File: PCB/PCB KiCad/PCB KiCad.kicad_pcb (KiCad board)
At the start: 2 copper layers, 40 x 40 mm, 54 parts, among them J1 Conn_01x04, J2 Qwiic, J3 Conn_01x04, J4 Conn_01x04, J5 Conn_01x04, U1 OPA2376AID, U2 NAU7802SGI, U3 TLC59208FIPWR, U4 LP5951MFX-1.8_NOPB

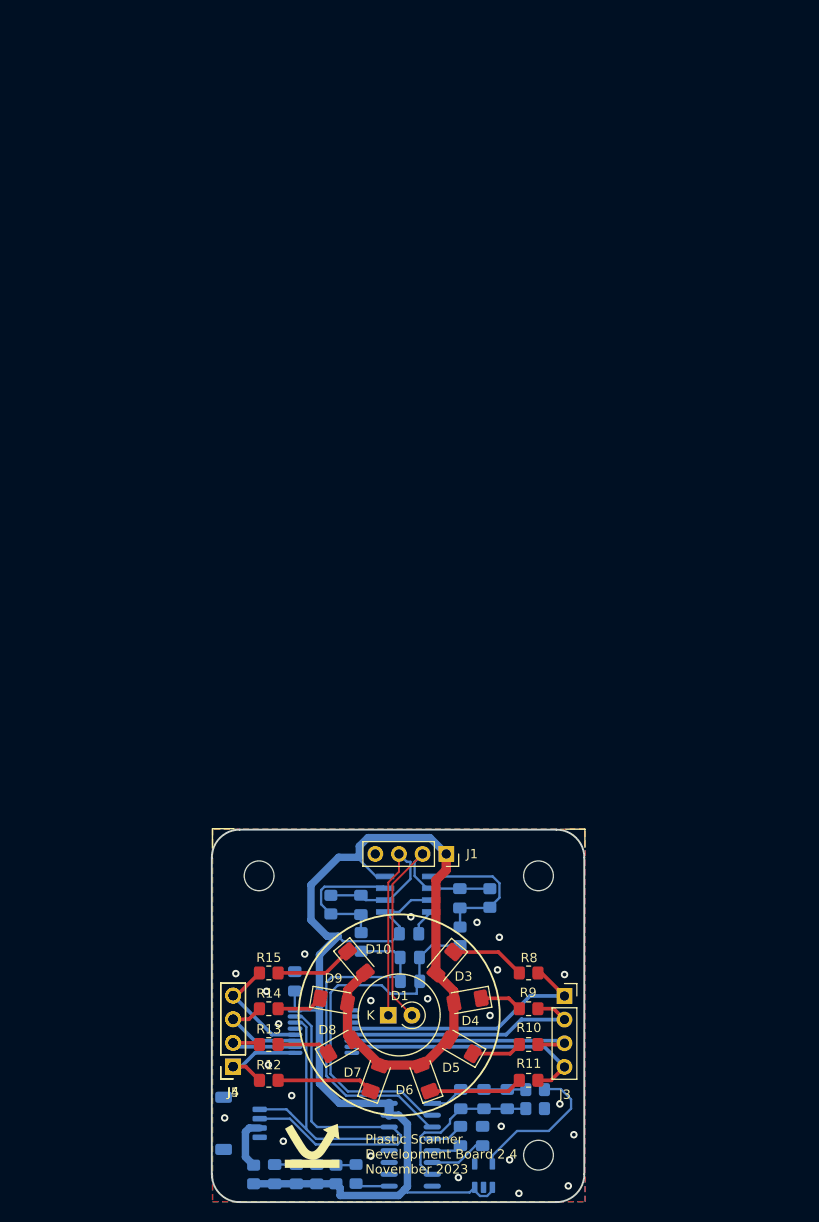
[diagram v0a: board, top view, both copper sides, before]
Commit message: Minor schematic cleanup!
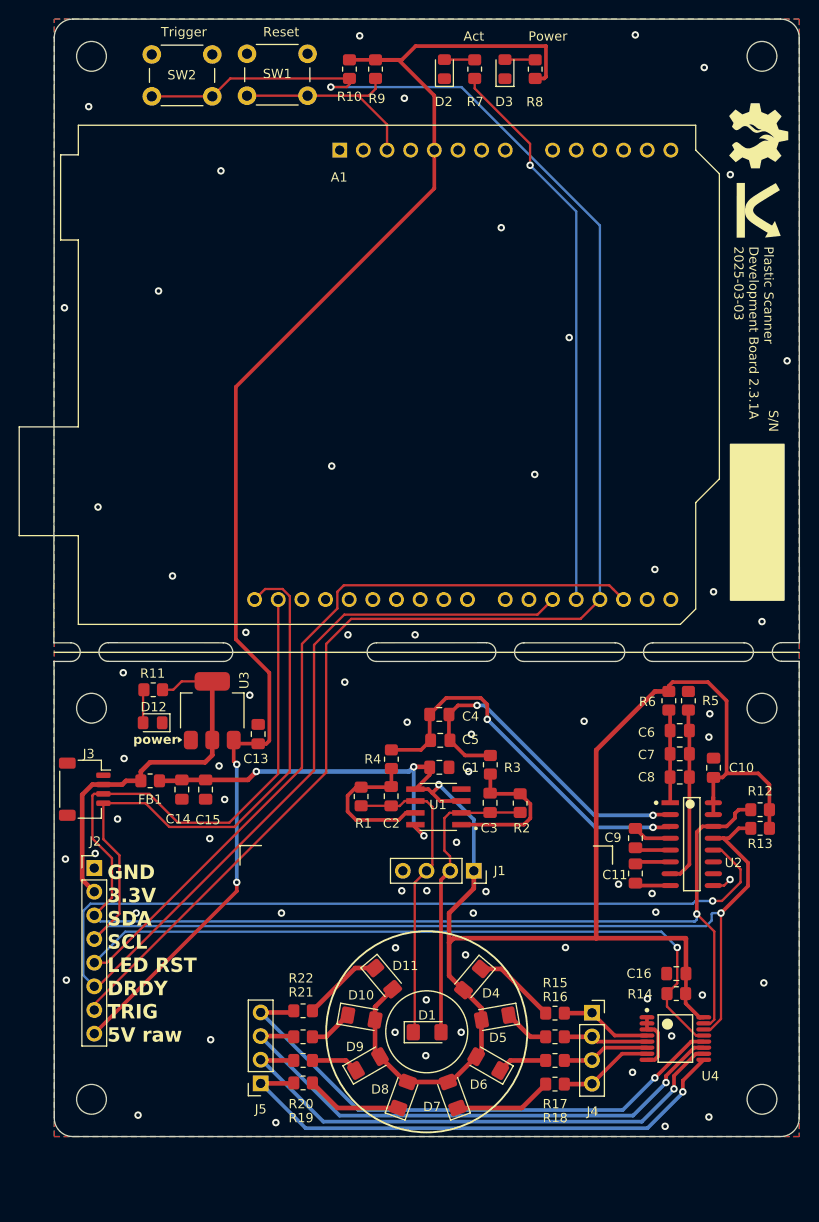
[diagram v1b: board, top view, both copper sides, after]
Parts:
- removed the C14 at (68.8, 131.3)
- removed the D10 at (75.4, 129.3)
- removed H1, H2, H4: MountingHole, MountingHole:MountingHole_3.2mm_M3
- removed the J4 at (62.2, 140.5)
- removed the R11 at (93.9, 142.0)
- removed the R15 at (66.0, 130.4)
- added ?: MountingHole_3.2mm_M3, MountingHole:MountingHole_3.2mm_M3, F.Cu at (119.0, 32.0)
- added ?: MountingHole_3.2mm_M3, MountingHole:MountingHole_3.2mm_M3, F.Cu at (47.0, 144.0)
- added A1: Arduino_UNO_R3, Module:Arduino_UNO_R3, F.Cu at (73.7, 42.1)
- added C15: 22u, Capacitor_SMD:C_0805_2012Metric_Pad1.18x1.45mm_HandSolder, F.Cu at (59.2, 110.7)
- added C16: 100n, Capacitor_SMD:C_0805_2012Metric_Pad1.18x1.45mm_HandSolder, F.Cu at (109.8, 130.5)
- added D11: 1720nm, LED_SMD:LED_1206_3216Metric_Pad1.42x1.75mm_HandSolder, F.Cu at (78.4, 131.0)
- added D12: LED RED, LED_SMD:LED_0805_2012Metric_Pad1.15x1.40mm_HandSolder, F.Cu at (53.6, 103.6)
- added D3: LED RED, LED_SMD:LED_0805_2012Metric_Pad1.15x1.40mm_HandSolder, F.Cu at (91.4, 33.4)
- added G***: LOGO, LOGO, F.Cu at (118.9, 48.5)
- added G***: LOGO, LOGO, F.Cu at (118.6, 40.5)
- added G***: LOGO, LOGO, B.Cu at (83.4, 121.0)
- added G1: LOGO, LOGO, B.Cu at (82.0, 66.0)
- added J2: Conn_01x08, Connector_PinHeader_2.54mm:PinHeader_1x08_P2.54mm_Vertical, F.Cu at (47.3, 119.2)
- added R16: 47, Resistor_SMD:R_0805_2012Metric_Pad1.20x1.40mm_HandSolder, F.Cu at (96.8, 137.3)
- added R17: 47, Resistor_SMD:R_0805_2012Metric_Pad1.20x1.40mm_HandSolder, F.Cu at (96.8, 139.8)
- added R18: 47, Resistor_SMD:R_0805_2012Metric_Pad1.20x1.40mm_HandSolder, F.Cu at (96.8, 142.4)
- added R19: 47, Resistor_SMD:R_0805_2012Metric_Pad1.20x1.40mm_HandSolder, F.Cu at (69.7, 142.2)
- added R20: 47, Resistor_SMD:R_0805_2012Metric_Pad1.20x1.40mm_HandSolder, F.Cu at (69.7, 139.8)
- added R21: 47, Resistor_SMD:R_0805_2012Metric_Pad1.20x1.40mm_HandSolder, F.Cu at (69.7, 137.3)
- added R22: 47, Resistor_SMD:R_0805_2012Metric_Pad1.20x1.40mm_HandSolder, F.Cu at (69.7, 134.5)
- added R7: 100, Resistor_SMD:R_0805_2012Metric_Pad1.20x1.40mm_HandSolder, F.Cu at (88.2, 33.4)
- added R8: 100, Resistor_SMD:R_0805_2012Metric_Pad1.20x1.40mm_HandSolder, F.Cu at (94.7, 33.4)
- added REF**: MountingHole_3.2mm_M3, MountingHole:MountingHole_3.2mm_M3, F.Cu at (47.0, 32.0)
- added SW1: MCU_RESET, Button_Switch_THT:SW_PUSH_6mm, F.Cu at (63.7, 31.7)
- added SW2: TRIGGER, Button_Switch_THT:SW_PUSH_6mm, F.Cu at (53.5, 31.8)
- added e: MountingHole_3.2mm_M3, MountingHole:MountingHole_3.2mm_M3, F.Cu at (47.0, 102.0)
- added e: MountingHole_3.2mm_M3, MountingHole:MountingHole_3.2mm_M3, F.Cu at (119.0, 144.0)
- added e: MountingHole_3.2mm_M3, MountingHole:MountingHole_3.2mm_M3, F.Cu at (119.0, 102.0)
- C1, C10, C11, C2, C3, C4, C5, C6, C7, C8, C9, FB1, R1, R2, R3, R4, R5, R6, U1, U2: moved to F.Cu
- C13: value 22u -> 10u; moved to F.Cu
- C14: renamed from C12; moved to F.Cu
- D1: footprint Diode_THT:D_A-405_P2.54mm_Vertical_KathodeUp -> Diode_SMD:D_1206_3216Metric_Pad1.42x1.75mm_HandSolder
- D2: value LED RED -> LED BLUE; moved to F.Cu
- G***: moved to B.Cu
- J3: renamed from J2; moved to F.Cu
- R10, R9: value 47 -> 10k
- R11: renamed from R7; moved to F.Cu
- R12, R13: value 47 -> 4.7k
- R14: value 47 -> 1k
- U3: value TLC59208FIPWR -> AMS1117-3.3; footprint TLC59208:Texas_Instruments-TLC59208FIPWR-Level_A -> Package_TO_SOT_SMD:SOT-223-3_TabPin2; moved to F.Cu
- U4: value LP5951MFX-1.8_NOPB -> TLC59208FIPWR; footprint LP5951MFX-1.8_NOPB:SOT95P280X145-5N -> TLC59208:Texas_Instruments-TLC59208FIPWR-Level_A; moved to F.Cu
- moved D2 119.0 mm to (84.9, 33.4)
- moved R10 106.5 mm to (74.7, 33.4), turned to -90 degrees
- moved R9 102.2 mm to (77.5, 33.4), turned to -90 degrees
- moved C10 64.2 mm to (113.8, 108.4)
- moved R12 60.2 mm to (118.8, 112.9), turned to 180 degrees
- moved R13 57.6 mm to (118.8, 114.9), turned to 180 degrees
- moved R11 55.6 mm to (53.6, 100.0), turned to 180 degrees
- moved G*** 52.4 mm to (98.1, 104.1), turned to 180 degrees
- moved C13 47.4 mm to (64.9, 104.8)
- moved G*** 47.2 mm to (106.4, 104.3)
- moved R5 46.8 mm to (111.1, 101.2), turned to 90 degrees
- moved U2 44.2 mm to (111.5, 116.6), turned to 0 degrees
- moved R6 44.2 mm to (109.0, 101.2), turned to 90 degrees
- moved R14 43.8 mm to (109.8, 132.7)
- moved C14 43.8 mm to (56.7, 110.7), turned to 90 degrees
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- renumbered D9 to D10, D3 to D4, D4 to D5, D5 to D6, D6 to D7, D7 to D8, D8 to D9, J3 to J4, R8 to R15
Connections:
- C1 pad 2: 3.3v -> +3.3V
- C10 pad 1: 3.3v -> +3.3V
- C13 pad 1: 3.3v -> 5v_RAW
- C14 pad 2: 3.3v -> +3.3V
- D10 pad 1: Net-(D9-K) -> Net-(D10-K)
- D10 pad 2: 3.3v -> +3.3V
- D4 pad 2: 3.3v -> +3.3V
- D5 pad 1: Net-(D4-K) (its old number) -> Net-(D5-K)
- D5 pad 2: 3.3v -> +3.3V
- D6 pad 1: Net-(D5-K) -> Net-(D6-K)
- D6 pad 2: 3.3v -> +3.3V
- D7 pad 2: 3.3v -> +3.3V
- D8 pad 1: Net-(D7-K) (its old number) -> Net-(D8-K)
- D8 pad 2: 3.3v -> +3.3V
- D9 pad 1: Net-(D8-K) -> Net-(D9-K)
- D9 pad 2: 3.3v -> +3.3V
- FB1 pad 1: 3.3v -> +3.3V
- J1 pad 1: 3.3v -> +3.3V
- R10 pad 1: LED3 -> 5v_RAW
- R10 pad 2: Net-(D5-K) -> TRIGGER
- R11 pad 1: 3.3v -> 3v3unf
- R11 pad 2: Net-(D2-A) -> Net-(D12-A)
- R12 pad 1: LED5 -> +3.3V
- R12 pad 2: Net-(D7-K) (its old number) -> SDA
- R13 pad 1: LED6 -> +3.3V
- R13 pad 2: Net-(D8-K) -> SCL
- R14 pad 1: LED7 -> LED_RESET
- R14 pad 2: Net-(D9-K) -> +3.3V
- R6 pad 2: Net-(U4-VOUT) -> +3.3V
- R9 pad 1: LED2 -> 5v_RAW
- R9 pad 2: Net-(D4-K) (its old number) -> MCU_RESET
- U1 pad 3: 3.3v -> +3.3V
- U1 pad 5: 3.3v -> +3.3V
- U1 pad 8: 3.3v -> +3.3V
- U2 pad 12: unconnected-(U2-DRDY-Pad12) -> DRDY_INT
- U2 pad 15: 3.3v -> +3.3V
- U2 pad 16: 3.3v -> +3.3V
- U3 pad 2: GND -> 3v3unf
- U3 pad 3: GND -> 5v_RAW
- U4 pad 1: 3.3v -> GND
- U4 pad 3: 3.3v -> GND
- U4 pad 4: (no net) -> LED1
- U4 pad 5: Net-(U4-VOUT) -> LED2
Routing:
- net +3.3V: track 0.00 -> 200.4 mm, vias 0 -> 4
- net TRIGGER: track 0.00 -> 181.0 mm, vias 0 -> 1
- net DRDY_INT: track 0.00 -> 159.9 mm, vias 0 -> 1
- net LED_RESET: track 0.00 -> 159.8 mm, vias 0 -> 1
- net 3.3v: track 156.1 -> 0.00 mm
- net 5v_RAW: track 0.00 -> 155.9 mm, vias 0 -> 2
- net SCL: track 27.6 -> 160.7 mm, vias 0 -> 1
- net SDA: track 39.7 -> 151.7 mm, vias 0 -> 1
- net LED_BLUE: track 0.00 -> 60.5 mm, vias 0 -> 1
- net LED6: track 9.73 -> 57.8 mm, vias 0 -> 1
- net LED7: track 10.9 -> 58.2 mm, vias 0 -> 1
- net LED8: track 12.2 -> 58.6 mm, vias 0 -> 1
- net LED5: track 10.7 -> 56.9 mm, vias 0 -> 1
- net 3v3unf: track 5.64 -> 40.9 mm
- net MCU_RESET: track 0.00 -> 22.3 mm
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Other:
- board size 40 x 40 mm -> 80.1 x 120 mm
- board text added: "Act"
- board text added: "GND 3.3V SDA SCL LED RST DRDY TRIG 5V raw"
- board text added: "Plastic Scanner Development Board 2.3 May 2023"
- board text added: "Plastic Scanner Development Board 2.3.1A 2025-03-03"
- board text added: "Power"
- board text added: "Reset"
- board text added: "S/N"
- board text added: "Trigger"
- board text removed: "Plastic Scanner Development Board 2.4 November 2023"
